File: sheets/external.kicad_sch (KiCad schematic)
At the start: 18 parts, among them CN2 StemmaQT, J10 USART3, J11 UART8, J12 Conn_01x03_Pin, J13 Conn_01x06_Pin, J14 Conn_01x05_Pin, J15 Conn_01x03_Pin, J16 Conn_01x06_Pin, J17 Conn_01x05_Pin, J3 Airbrake_Pot2, J4 Airbrake_Pot1, J5 SPARE_ADC2, J6 PWM1, J7 SPARE_ADC1, J8 Conn_01x04_Pin, J9 PWM2

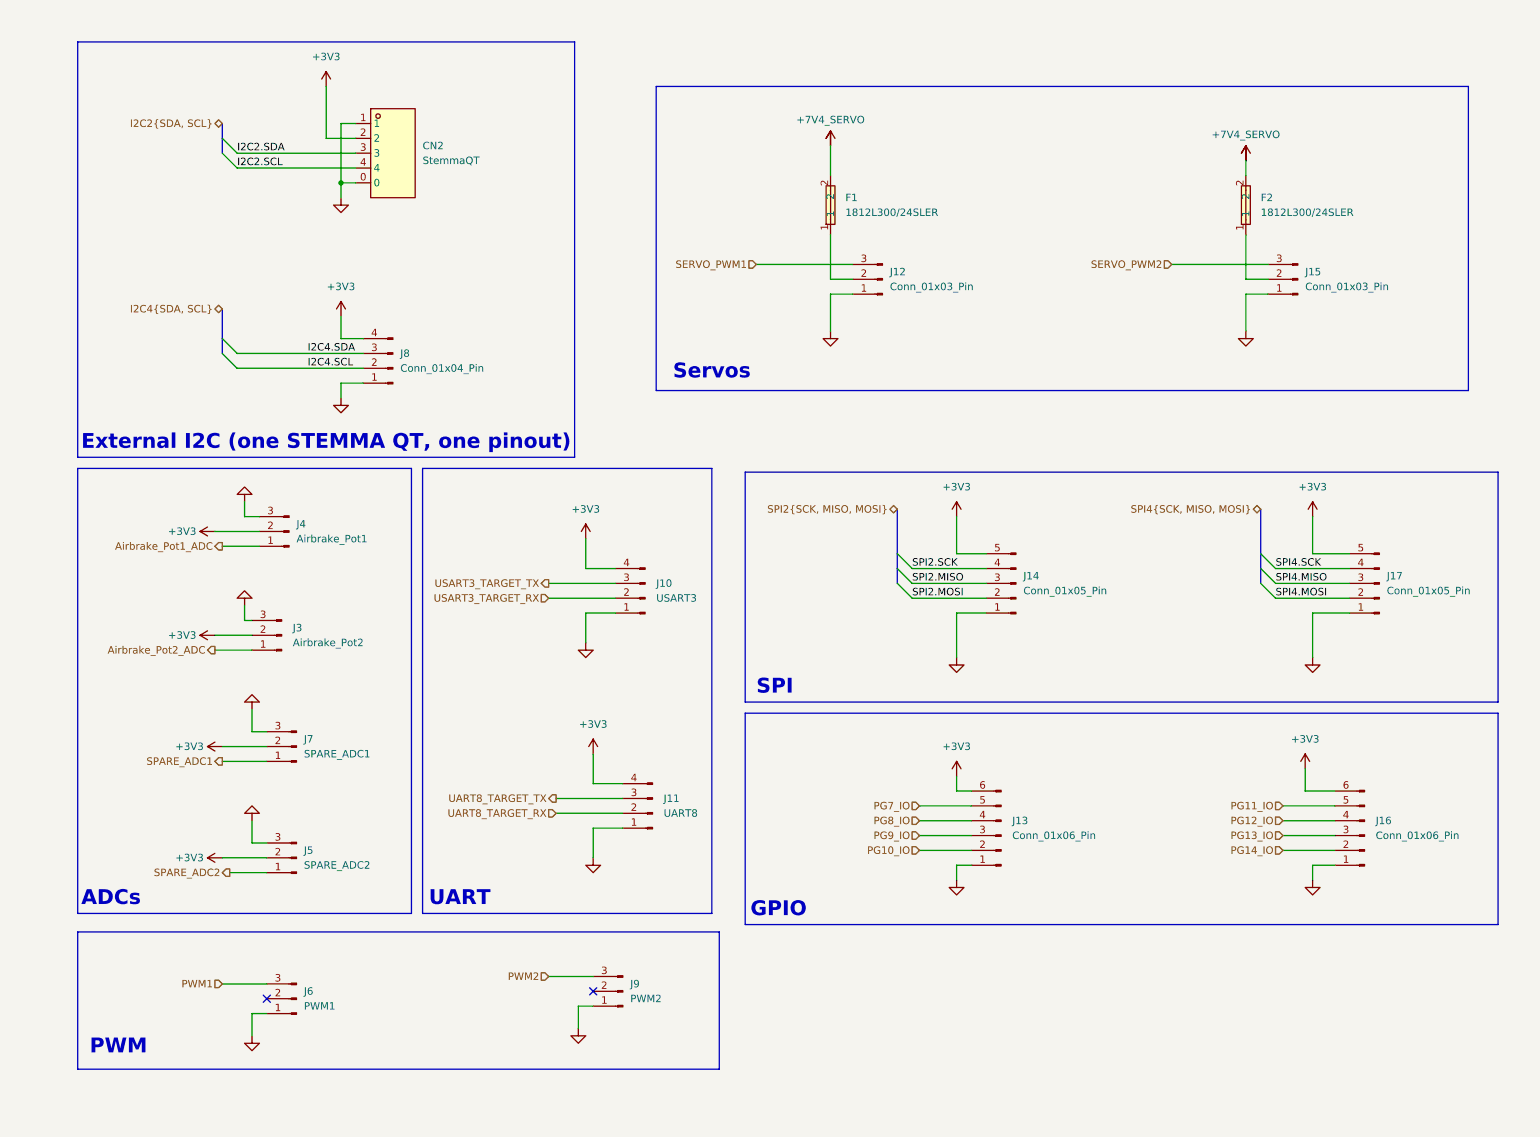
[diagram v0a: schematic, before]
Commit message: some changes for 2027 aerolotl
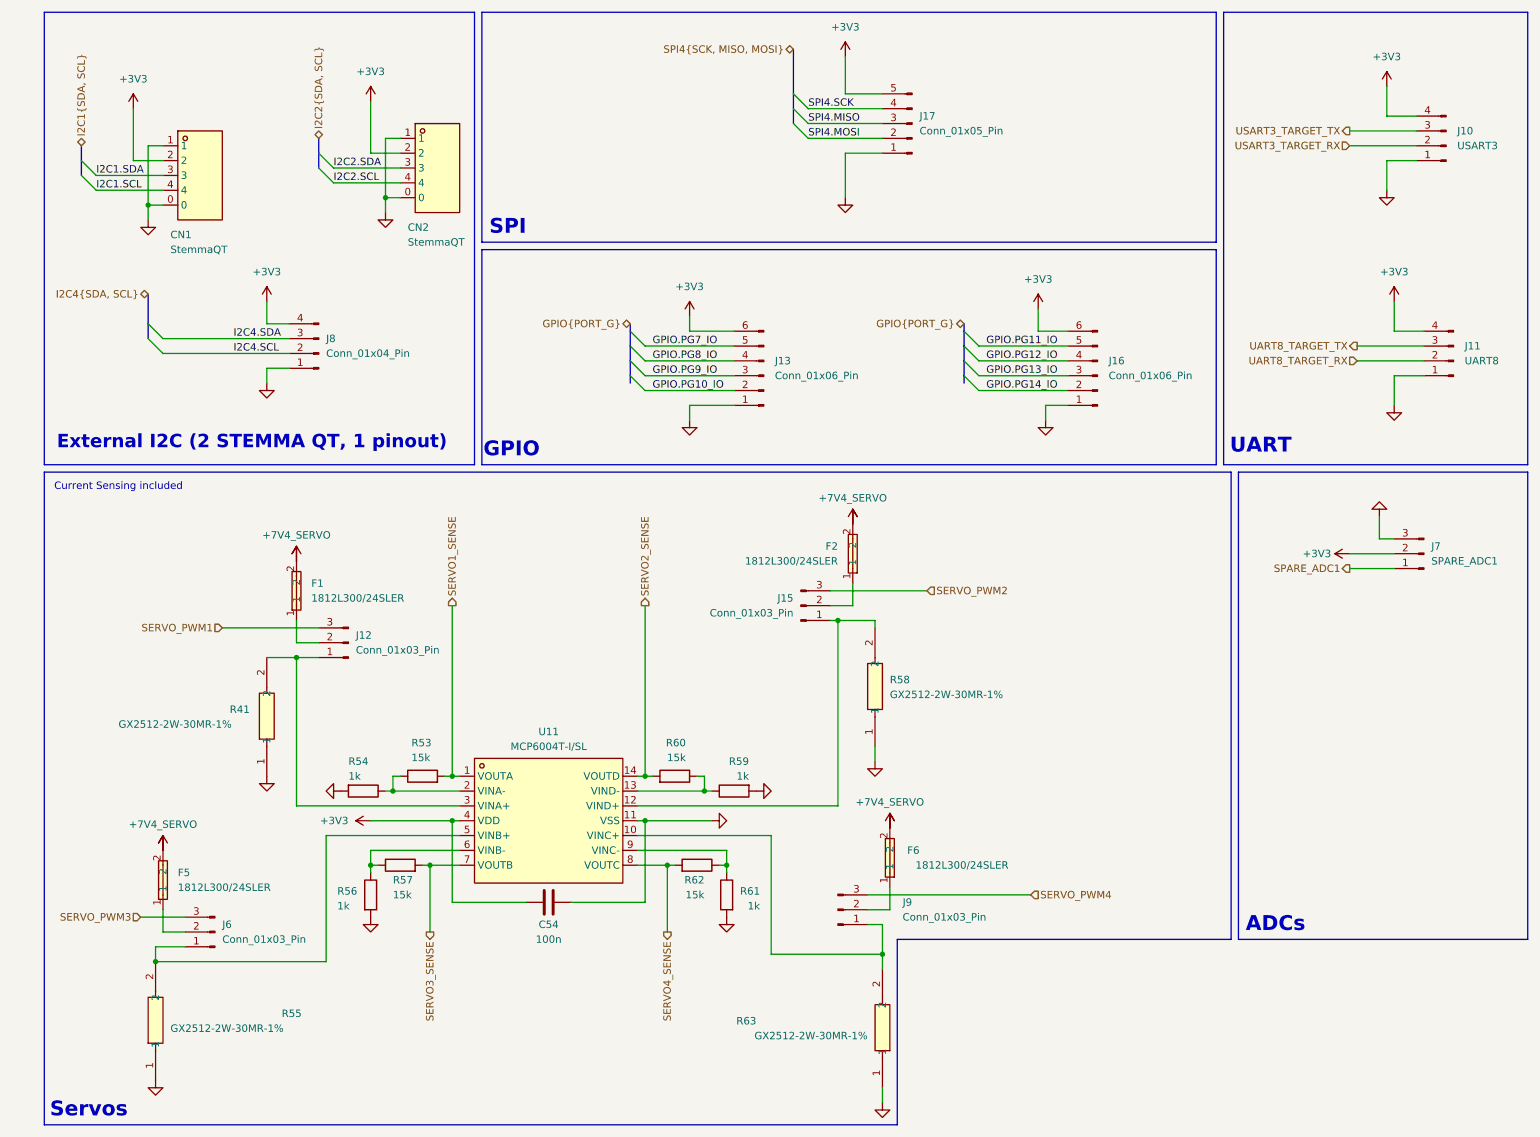
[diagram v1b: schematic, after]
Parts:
- removed J14: Conn_01x05_Pin, symbol Connector:Conn_01x05_Pin
- removed J3: Airbrake_Pot2, symbol Connector:Conn_01x03_Pin
- removed J4: Airbrake_Pot1, symbol Connector:Conn_01x03_Pin
- removed J5: SPARE_ADC2, symbol Connector:Conn_01x03_Pin
- added C54: 100n, symbol Device:C
- added CN1: StemmaQT, aerolotl_custom:CONN-SMD_BM04B-SRSS-TB, symbol aerolotl_custom:StemmaQT
- added F5, F6: 1812L300/24SLER, Capacitor_SMD:C_0402_1005Metric, symbol aerolotl_custom:1812L300_24SLER
- added R41, R55, R58, R63: GX2512-2W-30MR-1%, aerolotl_custom:RES-SMD_L6.4-W3.2-1, symbol aerolotl_custom:GX2512-2W-30MR-1%
- added R53, R57, R60, R62: 15k, symbol Device:R
- added R54, R56, R59, R61: 1k, symbol Device:R
- added U11: MCP6004T-I/SL, aerolotl_custom:SOIC-14_L8.7-W3.9-P1.27-LS6.0-BL, symbol aerolotl_custom:MCP6004T-I_SL
- F2: footprint aerolotl_custom:F1812 -> Capacitor_SMD:C_0402_1005Metric
- J6: value PWM1 -> Conn_01x03_Pin
- J9: value PWM2 -> Conn_01x03_Pin
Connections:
- net +3V3: now also C54.1, CN1.2, U11.4 (VDD)
- net +7V4_SERVO: now also F5.2, F6.2
- net GND: now also C54.2, CN1.0, CN1.1, R41.1, R54.2, R55.1, R56.2, R58.1, R59.2, R61.2, R63.1, U11.11 (VSS); no longer J12.1 (Pin_1), J15.1 (Pin_1), J6.1 (Pin_1), J9.1 (Pin_1)
- net at J9.2 (Pin_2): now also F6.1
- net at J6.2 (Pin_2): now also F5.1
- net PG10_IO renamed GPIO.PG10_IO
- net PG11_IO renamed GPIO.PG11_IO
- net PG12_IO renamed GPIO.PG12_IO
- net PG13_IO renamed GPIO.PG13_IO
- net PG14_IO renamed GPIO.PG14_IO
- net PG7_IO renamed GPIO.PG7_IO
- net PG8_IO renamed GPIO.PG8_IO
- net PG9_IO renamed GPIO.PG9_IO
- net PWM1 renamed SERVO_PWM3
- net PWM2 renamed SERVO_PWM4
- new net: J15.1 (Pin_1), R58.2, U11.12 (VIND+)
- new net: R59.1, R60.1, U11.13 (VIND-)
- new net: R56.1, R57.1, U11.6 (VINB-)
- new net: J9.1 (Pin_1), R63.2, U11.10 (VINC+)
- new net: R53.1, R54.1, U11.2 (VINA-)
- new net: J12.1 (Pin_1), R41.2, U11.3 (VINA+)
- new net: J6.1 (Pin_1), R55.2, U11.5 (VINB+)
- new net: R61.1, R62.1, U11.9 (VINC-)
- new net I2C1.SCL: CN1.4
- new net I2C1.SDA: CN1.3
- new net SERVO1_SENSE: R53.2, U11.1 (VOUTA)
- new net SERVO2_SENSE: R60.2, U11.14 (VOUTD)
- new net SERVO3_SENSE: R57.2, U11.7 (VOUTB)
- new net SERVO4_SENSE: R62.2, U11.8 (VOUTC)
- no-connect marks 2 -> 0
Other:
- note added: "Current Sensing included"
- note added: "External I2C (2 STEMMA QT, 1 pinout)"
- note removed: "External I2C (one STEMMA QT, one pinout)"
- note removed: "PWM"
- moved on the sheet: CN2, F1, J10, J11, J12, J13, J16, J17, J7, J8
